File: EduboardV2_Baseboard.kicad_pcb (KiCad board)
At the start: 2 copper layers, 2 parts, among them IC301 XL1509-5.0E1, X201 PCIE-52P40H

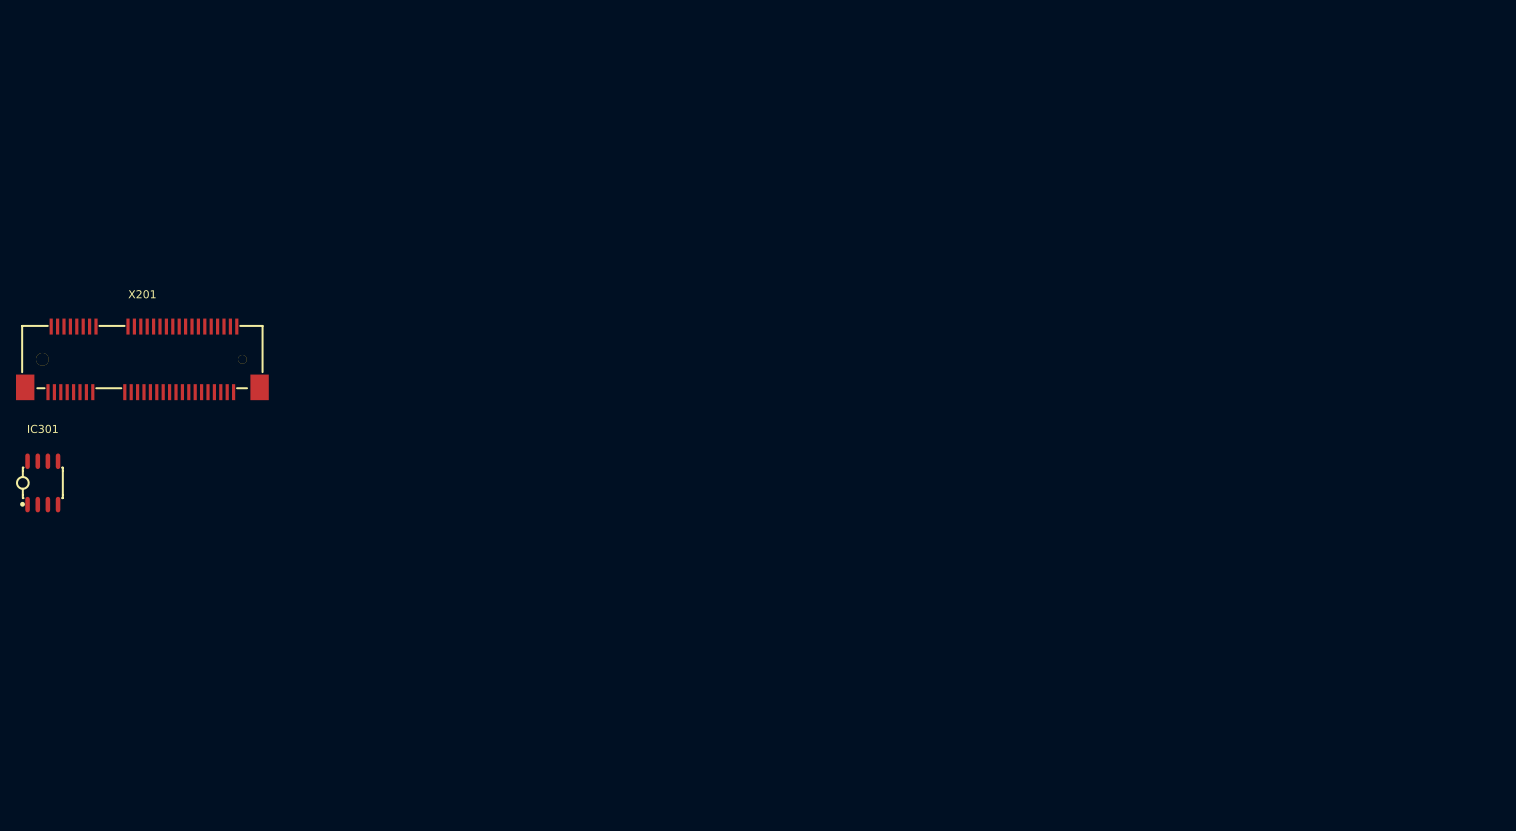
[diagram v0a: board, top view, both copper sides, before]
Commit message: added more components
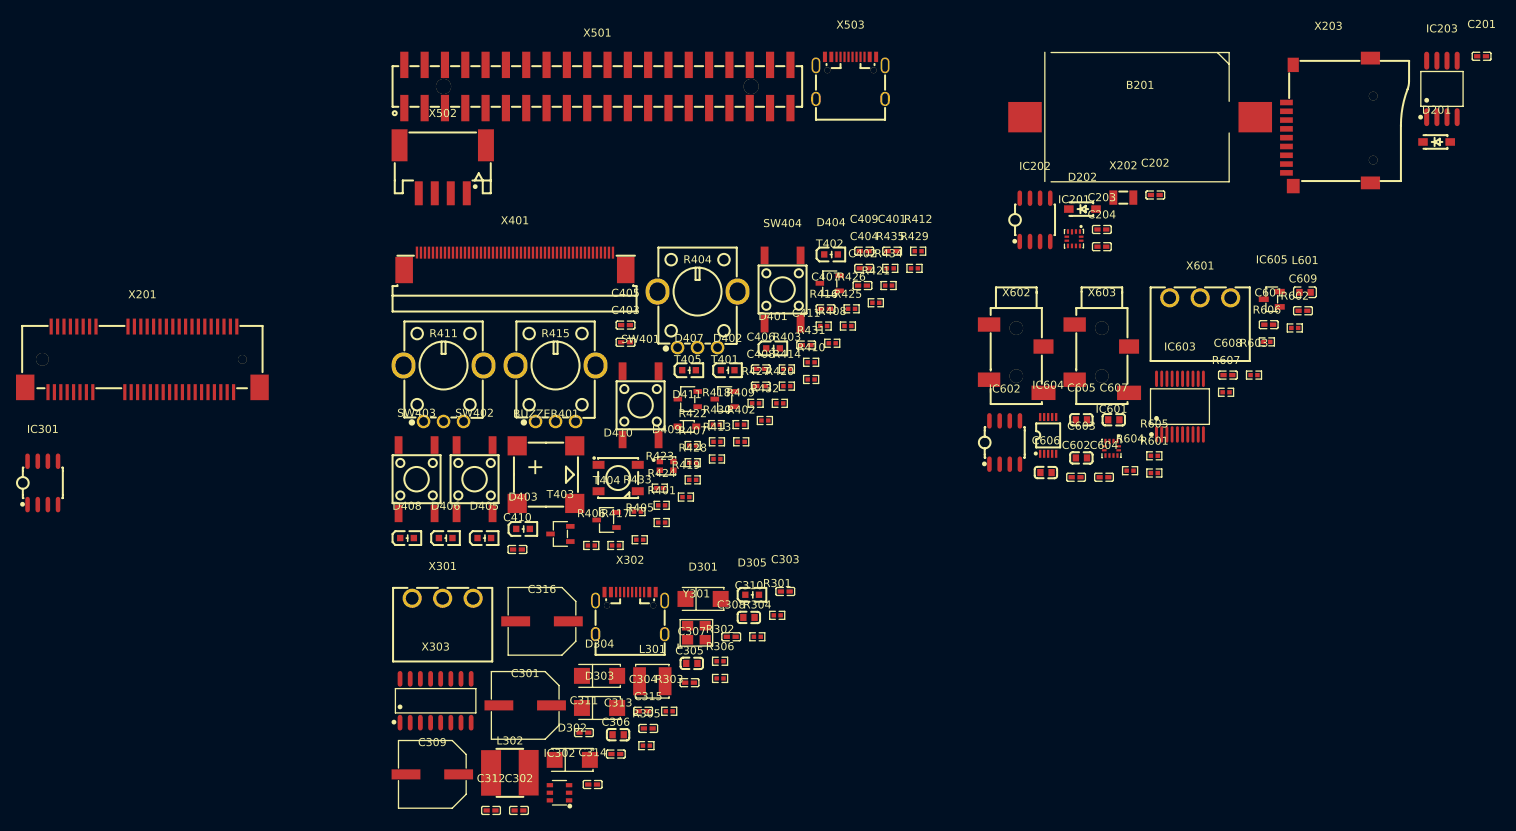
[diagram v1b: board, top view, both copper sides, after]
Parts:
- added B201: CR2032-BS-6-1, eduboardv2:BAT-TH_CR2032-BS-6-1, F.Cu at (213.4, 35.6)
- added BUZZER401: MLT-8530, eduboardv2:BUZ-SMD_4P-L8.5-W8.5-P8.50-TL, F.Cu at (139.1, 80.2)
- added C201: 10pF, eduboardv2:C0402, F.Cu at (256.0, 27.9)
- added C202: 1uF, eduboardv2:C0402, F.Cu at (215.3, 45.3)
- added C203: 10nF, eduboardv2:C0402, F.Cu at (208.6, 49.6)
- added C204: 100nF, eduboardv2:C0402, F.Cu at (208.6, 51.8)
- added C301: 220uF, 35V, eduboardv2:CAP-SMD_BD8.0-L8.3-W8.3-RD, F.Cu at (136.5, 109.1)
- added C302: 100nF, 50V, eduboardv2:C0402, F.Cu at (135.7, 122.2)
- added C303: 22pF, eduboardv2:C0402, F.Cu at (169.0, 94.8)
- added C304: 22pF, eduboardv2:C0402, F.Cu at (151.2, 109.8)
- added C305: 100nF, 50V, eduboardv2:C0402, F.Cu at (157.0, 106.2)
- added C306: 100nF, 50V, eduboardv2:C0402, F.Cu at (147.8, 115.2)
- added C307: 10uF, X5R, 25V, eduboardv2:C0603, F.Cu at (157.3, 103.8)
- added C308: 22pF, eduboardv2:C0402, F.Cu at (162.2, 100.5)
- added C309: 220uF, 35V, eduboardv2:CAP-SMD_BD8.0-L8.3-W8.3-RD, F.Cu at (124.9, 117.7)
- added C310: 10uF, X5R, 25V, eduboardv2:C0603, F.Cu at (164.5, 98.1)
- added C311: 100nF, 50V, eduboardv2:C0402, F.Cu at (143.8, 112.5)
- added C312: 1uF, 25V, eduboardv2:C0402, F.Cu at (132.2, 122.2)
- added C313: 10uF, X5R, 25V, eduboardv2:C0603, F.Cu at (148.1, 112.8)
- added C314: 100nF, 50V, eduboardv2:C0402, F.Cu at (144.9, 119.0)
- added C315: 1uF, 25V, eduboardv2:C0402, F.Cu at (151.9, 112.0)
- added C316: 220uF, 35V, eduboardv2:CAP-SMD_BD8.0-L8.3-W8.3-RD, F.Cu at (138.6, 98.6)
- added C401: 1nF, eduboardv2:C0402, F.Cu at (182.4, 52.3)
- added C402: 10nF, eduboardv2:C0402, F.Cu at (178.7, 56.6)
- added C403: 1nF, eduboardv2:C0402, F.Cu at (149.0, 63.7)
- added C404: 10nF, eduboardv2:C0402, F.Cu at (178.9, 54.5)
- added C405: 1nF, eduboardv2:C0402, F.Cu at (149.0, 61.5)
- added C406: 10nF, eduboardv2:C0402, F.Cu at (165.9, 67.0)
- added C407: 100nF, eduboardv2:C0402, F.Cu at (174.0, 59.5)
- added C408: 10nF, eduboardv2:C0402, F.Cu at (165.9, 69.2)
- added C409: 100nF, eduboardv2:C0402, F.Cu at (178.9, 52.3)
- added C410: 1uF, eduboardv2:C0402, F.Cu at (135.5, 89.6)
- added C411: 1uF, eduboardv2:C0402, F.Cu at (171.6, 64.0)
- added C601: 100nF, eduboardv2:C0402, F.Cu at (229.4, 61.5)
- added C602: 100nF, eduboardv2:C0402, F.Cu at (205.4, 80.6)
- added C603: 10uF, eduboardv2:C0603, F.Cu at (206.0, 78.2)
- added C604: 100nF, eduboardv2:C0402, F.Cu at (208.8, 80.6)
- added C605: 10uF, eduboardv2:C0603, F.Cu at (206.0, 73.4)
- added C606: 4.7uF, eduboardv2:C0603, F.Cu at (201.6, 80.0)
- added C607: 4.7uF, eduboardv2:C0603, F.Cu at (210.1, 73.4)
- added C608: 2.2nF, eduboardv2:C0402, F.Cu at (224.3, 67.8)
- added C609: 2.2nF, eduboardv2:C0402, F.Cu at (233.7, 59.8)
- added D201: B5819W_C8598, eduboardv2:SOD-123_L2.7-W1.6-LS3.7-RD-1, F.Cu at (250.4, 38.7)
- added D202: B5819W_C8598, eduboardv2:SOD-123_L2.7-W1.6-LS3.7-RD-1, F.Cu at (206.2, 47.0)
- added D301: SS210, eduboardv2:SMA_L4.3-W2.6-LS5.2-RD, F.Cu at (158.7, 95.8)
- added D302: SS210, eduboardv2:SMA_L4.3-W2.6-LS5.2-RD, F.Cu at (142.4, 115.9)
- added D303: SS210, eduboardv2:SMA_L4.3-W2.6-LS5.2-RD, F.Cu at (145.8, 109.4)
- added D304: SS210, eduboardv2:SMA_L4.3-W2.6-LS5.2-RD, F.Cu at (145.8, 105.4)
- added D305: blue, eduboardv2:LED0603-R-RD_BLUE, F.Cu at (164.9, 95.3)
- added D401: blue, eduboardv2:LED0603-R-RD_BLUE, F.Cu at (167.5, 64.5)
- added D402: blue, eduboardv2:LED0603-R-RD_BLUE, F.Cu at (161.8, 67.2)
- added D403: blue, eduboardv2:LED0603-R-RD_BLUE, F.Cu at (136.2, 87.0)
- added D404: blue, eduboardv2:LED0603-R-RD_BLUE, F.Cu at (174.7, 52.7)
- added D405: blue, eduboardv2:LED0603-R-RD_BLUE, F.Cu at (131.4, 88.2)
- added D406: blue, eduboardv2:LED0603-R-RD_BLUE, F.Cu at (126.6, 88.2)
- added D407: blue, eduboardv2:LED0603-R-RD_BLUE, F.Cu at (157.0, 67.2)
- added D408: blue, eduboardv2:LED0603-R-RD_BLUE, F.Cu at (121.7, 88.2)
- added D409: RGB-LED, eduboardv2:LED-SMD_FM-B2020RGBA-HG, F.Cu at (154.2, 79.2)
- added D410: WS2812B-B_W, eduboardv2:LED-SMD_4P-L5.0-W5.0-TL_WS2812B-B, F.Cu at (148.1, 80.7)
- added D411: 1N4148WST4, eduboardv2:SOD-323_L1.8-W1.3-LS2.5-RD, F.Cu at (156.7, 74.2)
- added IC201: STK8321, eduboardv2:LGA-12_L2.0-W2.0-P0.50-TR, F.Cu at (205.1, 50.8)
- added IC202: PCF8563T_5,518, eduboardv2:SOIC-8_L5.0-W4.0-P1.27-LS6.0-BL, F.Cu at (200.2, 48.4)
- added IC203: W25Q128JVSIQTR, eduboardv2:SOIC-8_L5.3-W5.3-P1.27-LS8.0-BL, F.Cu at (251.1, 32.0)
- added IC302: SY8113BADC, eduboardv2:TSOT-23-6_L2.9-W1.6-P0.95-LS2.8-BR, F.Cu at (140.8, 120.0)
- added IC601: STK8321, eduboardv2:LGA-12_L2.0-W2.0-P0.50-TR, F.Cu at (209.8, 77.0)
- added IC602: SP3485EN-L_TR, eduboardv2:SOIC-8_L5.0-W4.0-P1.27-LS6.0-BL, F.Cu at (196.4, 76.2)
- added IC603: WM8782SEDS_RV_C323842, eduboardv2:SSOP-20_L7.5-W5.2-P0.65-LS8.0-BL, F.Cu at (218.3, 71.7)
- added IC604: CS4344-CZZ, eduboardv2:TSSOP-10_L3.0-W3.0-P0.50-LS4.9-BL, F.Cu at (201.9, 75.3)
- added IC605: MCP9700AT-E_TT, eduboardv2:SOT-23-3_L2.9-W1.3-P1.90-LS2.4-BR, F.Cu at (229.8, 58.3)
- added L301: 6.8uH, 1A, eduboardv2:IND-SMD_L4.0-W4.0, F.Cu at (152.4, 106.1)
- added L302: 68uH, 1A, eduboardv2:IND-SMD_L6.0-W6.0_FNR60XXS, F.Cu at (134.6, 117.5)
- added L601: GZ1608D601TF, eduboardv2:L0603, F.Cu at (234.0, 57.5)
- added R301: 5.1k, eduboardv2:R0402, F.Cu at (168.0, 97.8)
- added R302: 5.1k, eduboardv2:R0402, F.Cu at (160.9, 103.6)
- added R303: 100k, eduboardv2:R0402, F.Cu at (154.5, 109.8)
- added R304: 22k, eduboardv2:R0402, F.Cu at (165.5, 100.5)
- added R305: 100k, eduboardv2:R0402, F.Cu at (151.6, 114.1)
- added R306: 1k, eduboardv2:R0402, F.Cu at (160.9, 105.7)
- added R401: 1k, eduboardv2:R0402, F.Cu at (153.6, 86.2)
- added R402: 10k, eduboardv2:R0402, F.Cu at (163.5, 76.1)
- added R403: 1k, eduboardv2:R0402, F.Cu at (169.2, 67.0)
- added R404: 50k, eduboardv2:RES-TH_RK09K1130AAU, F.Cu at (158.0, 60.9)
- added R405: 1k, eduboardv2:R0402, F.Cu at (150.8, 88.4)
- added R406: 1k, eduboardv2:R0402, F.Cu at (144.8, 89.1)
- added R407: 1k, eduboardv2:R0402, F.Cu at (157.4, 78.8)
- added R408: 1k, eduboardv2:R0402, F.Cu at (174.9, 63.8)
- added R409: 10k, eduboardv2:R0402, F.Cu at (163.4, 74.0)
- added R410: 1k, eduboardv2:R0402, F.Cu at (172.2, 68.3)
- added R411: 50k, eduboardv2:RES-TH_RK09K1130AAU, F.Cu at (126.3, 70.1)
- added R412: 1k, eduboardv2:R0402, F.Cu at (185.6, 52.3)
- added R413: 1k, eduboardv2:R0402, F.Cu at (160.5, 78.3)
- added R414: 1k, eduboardv2:R0402, F.Cu at (169.2, 69.2)
- added R415: 50k, eduboardv2:RES-TH_RK09K1130AAU, F.Cu at (140.3, 70.1)
- added R416: 1k, eduboardv2:R0402, F.Cu at (173.8, 61.7)
- added R417: 10k, eduboardv2:R0402, F.Cu at (147.8, 89.1)
- added R418: 150R, eduboardv2:R0402, F.Cu at (160.4, 74.0)
- added R419: 150R, eduboardv2:R0402, F.Cu at (156.6, 83.0)
- added R420: 1k, eduboardv2:R0402, F.Cu at (168.3, 71.3)
- added R421: 10k, eduboardv2:R0402, F.Cu at (180.3, 58.8)
- added R422: 150R, eduboardv2:R0402, F.Cu at (157.4, 76.6)
- added R423: 10R, eduboardv2:R0402, F.Cu at (153.3, 81.9)
- added R424: 10R, eduboardv2:R0402, F.Cu at (153.6, 84.1)
- added R425: 10R, eduboardv2:R0402, F.Cu at (176.8, 61.7)
- added R426: 10R, eduboardv2:R0402, F.Cu at (177.3, 59.5)
- added R427: 10R, eduboardv2:R0402, F.Cu at (165.3, 71.3)
- added R428: 10R, eduboardv2:R0402, F.Cu at (157.4, 80.9)
- added R429: NP, eduboardv2:R0402, F.Cu at (185.2, 54.5)
- added R430: 10R, eduboardv2:R0402, F.Cu at (160.5, 76.1)
- added R431: NP, eduboardv2:R0402, F.Cu at (172.2, 66.2)
- added R432: 10R, eduboardv2:R0402, F.Cu at (166.5, 73.5)
- added R433: 10R, eduboardv2:R0402, F.Cu at (150.5, 84.9)
- added R434: NP, eduboardv2:R0402, F.Cu at (181.9, 56.6)
- added R435: 10R, eduboardv2:R0402, F.Cu at (182.1, 54.5)
- added R601: 10k, eduboardv2:R0402, F.Cu at (215.1, 80.0)
- added R602: 120R, eduboardv2:R0402, F.Cu at (232.7, 61.9)
- added R603: 10k, eduboardv2:R0402, F.Cu at (227.6, 67.8)
- added R604: 10k, eduboardv2:R0402, F.Cu at (212.1, 79.8)
- added R605: 10k, eduboardv2:R0402, F.Cu at (215.1, 77.9)
- added R606: 470R, eduboardv2:R0402, F.Cu at (229.2, 63.6)
- added R607: 470R, eduboardv2:R0402, F.Cu at (224.1, 70.0)
- added SW401: K2-1102SP-C4SC-04, eduboardv2:KEY-SMD_4P-L6.0-W6.0-P4.50-LS9.5-BL, F.Cu at (150.9, 71.6)
- added SW402: K2-1102SP-C4SC-04, eduboardv2:KEY-SMD_4P-L6.0-W6.0-P4.50-LS9.5-BL, F.Cu at (130.2, 80.8)
- added SW403: K2-1102SP-C4SC-04, eduboardv2:KEY-SMD_4P-L6.0-W6.0-P4.50-LS9.5-BL, F.Cu at (122.9, 80.8)
- added SW404: K2-1102SP-C4SC-04, eduboardv2:KEY-SMD_4P-L6.0-W6.0-P4.50-LS9.5-BL, F.Cu at (168.7, 57.1)
- added T401: AO3400A, eduboardv2:SOT-23-3_L2.9-W1.6-P1.90-LS2.8-BR, F.Cu at (161.4, 70.8)
- added T402: AO3400A, eduboardv2:SOT-23-3_L2.9-W1.6-P1.90-LS2.8-BR, F.Cu at (174.6, 56.3)
- added T403: AO3400A, eduboardv2:SOT-23-3_L2.9-W1.6-P1.90-LS2.8-BR, F.Cu at (140.9, 87.7)
- added T404: AO3400A, eduboardv2:SOT-23-3_L2.9-W1.6-P1.90-LS2.8-BR, F.Cu at (146.7, 85.9)
- added T405: AO3400A, eduboardv2:SOT-23-3_L2.9-W1.6-P1.90-LS2.8-BR, F.Cu at (156.8, 70.8)
- added X202: 32.768 kHz, eduboardv2:FC-135R_L3.2-W1.5, F.Cu at (211.3, 45.6)
- added X203: TF-15×15, eduboardv2:TF-SMD_TF-15-15, F.Cu at (236.9, 36.2)
- added X301: KF2EDGR-3.81-3P, eduboardv2:CONN-TH_3P-P3.81_KF2EDGR-3.81-3P, F.Cu at (126.2, 95.7)
- added X302: USB3.1C16PFSMT, eduboardv2:USB-C-SMD_TYPE-C-USB-17, F.Cu at (149.6, 97.6)
- added X303: CH340G, eduboardv2:SOIC-16_L9.9-W3.9-P1.27-LS6.0-BL, F.Cu at (125.3, 108.5)
- added X401: ER-TFT035-6, eduboardv2:FPC-SMD_AFC07-S50ECA-00, F.Cu at (135.2, 53.6)
- added X501: PH-00650, eduboardv2:HDR-SMD_40P-P2.54-V-M-R2-C20-S7.8-EH, F.Cu at (145.5, 31.7)
- added X502: S4B-PH-SM4-K-TB(LF)(SN), eduboardv2:CONN-SMD_S4B-PH-SM4-K-TB-LF-SN, F.Cu at (126.2, 42.1)
- added X503: USB3.1C16PFSMT, eduboardv2:USB-C-SMD_TYPE-C-USB-17, F.Cu at (177.2, 30.7)
- added X601: KF2EDGR-3.81-3P, eduboardv2:CONN-TH_3P-P3.81_KF2EDGR-3.81-3P, F.Cu at (220.9, 58.1)
- added X602: PJ-327C-4A, eduboardv2:AUDIO-SMD_PJ-327C-4A, F.Cu at (197.9, 65.8)
- added X603: PJ-327C-4A, eduboardv2:AUDIO-SMD_PJ-327C-4A, F.Cu at (208.6, 65.8)
- added Y301: X322512MSB4SI, eduboardv2:OSC-SMD_4P-L3.2-W2.5-BL, F.Cu at (157.9, 100.0)
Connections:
- IC301 pad 1: unconnected-(IC301-Pad1) -> V_EXT
- IC301 pad 2: unconnected-(IC301-Pad2) -> Net-(IC301-Pad2)
- IC301 pad 3: unconnected-(IC301-Pad3) -> +5V_EXT
- IC301 pad 5: unconnected-(IC301-Pad5) -> GND
- IC301 pad 6: unconnected-(IC301-Pad6) -> GND
- IC301 pad 7: unconnected-(IC301-Pad7) -> GND
- IC301 pad 8: unconnected-(IC301-Pad8) -> GND
